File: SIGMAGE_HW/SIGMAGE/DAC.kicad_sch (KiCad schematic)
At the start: 80 parts, among them J20 SJ63073E, J21 SJ63073E, J24 SJ63073E, J25 SJ63073E, U10 PCM5102APWR, U20 PCM5102APWR, U21 PCM5102APWR, U3 PCM5102APWR

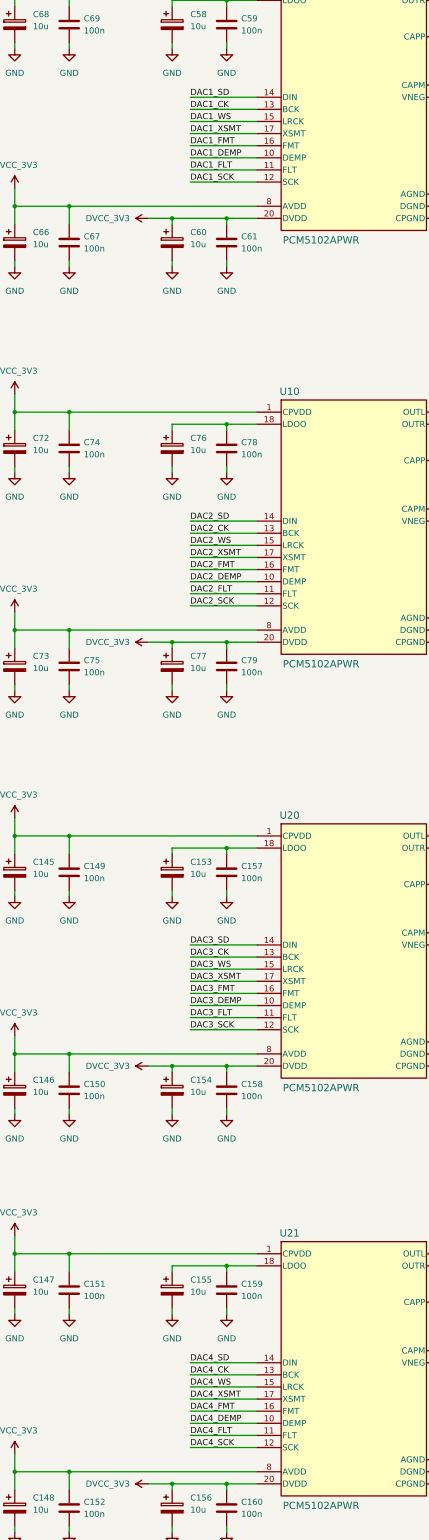
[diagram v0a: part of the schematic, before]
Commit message: finished schematic
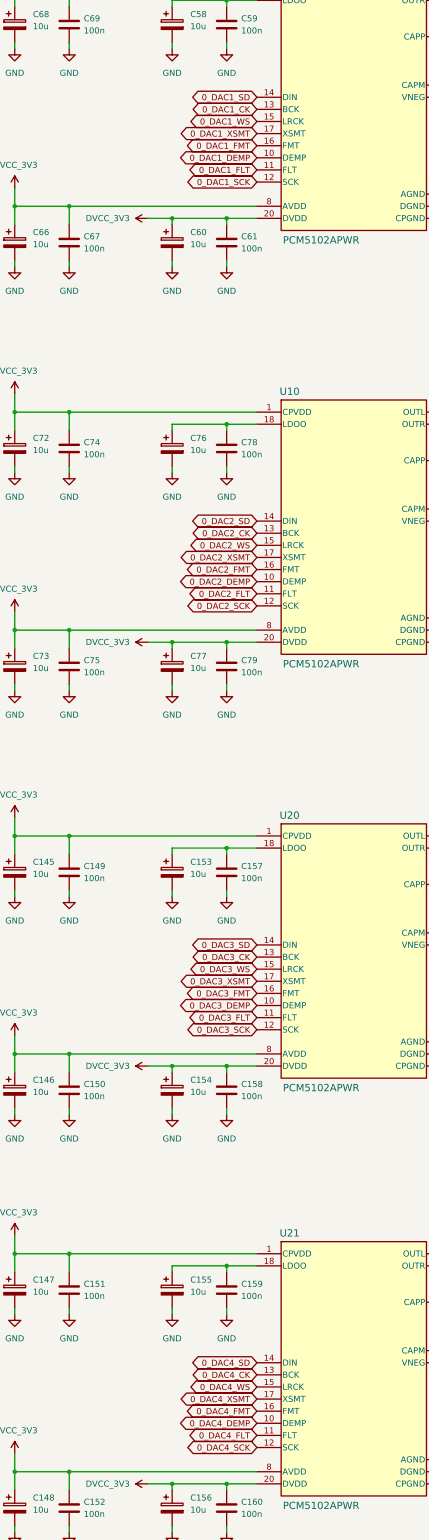
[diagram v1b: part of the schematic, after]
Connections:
- net DAC1_CK renamed 0_DAC1_CK
- net DAC1_DEMP renamed 0_DAC1_DEMP
- net DAC1_FLT renamed 0_DAC1_FLT
- net DAC1_FMT renamed 0_DAC1_FMT
- net DAC1_SCK renamed 0_DAC1_SCK
- net DAC1_SD renamed 0_DAC1_SD
- net DAC1_WS renamed 0_DAC1_WS
- net DAC1_XSMT renamed 0_DAC1_XSMT
- net DAC2_CK renamed 0_DAC2_CK
- net DAC2_DEMP renamed 0_DAC2_DEMP
- net DAC2_FLT renamed 0_DAC2_FLT
- net DAC2_FMT renamed 0_DAC2_FMT
- net DAC2_SCK renamed 0_DAC2_SCK
- net DAC2_SD renamed 0_DAC2_SD
- net DAC2_WS renamed 0_DAC2_WS
- net DAC2_XSMT renamed 0_DAC2_XSMT
- net DAC3_CK renamed 0_DAC3_CK
- net DAC3_DEMP renamed 0_DAC3_DEMP
- net DAC3_FLT renamed 0_DAC3_FLT
- net DAC3_FMT renamed 0_DAC3_FMT
- net DAC3_SCK renamed 0_DAC3_SCK
- net DAC3_SD renamed 0_DAC3_SD
- net DAC3_WS renamed 0_DAC3_WS
- net DAC3_XSMT renamed 0_DAC3_XSMT
- net DAC4_CK renamed 0_DAC4_CK
- net DAC4_DEMP renamed 0_DAC4_DEMP
- net DAC4_FLT renamed 0_DAC4_FLT
- net DAC4_FMT renamed 0_DAC4_FMT
- net DAC4_SCK renamed 0_DAC4_SCK
- net DAC4_SD renamed 0_DAC4_SD
- net DAC4_WS renamed 0_DAC4_WS
- net DAC4_XSMT renamed 0_DAC4_XSMT

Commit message: uga uga
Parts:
- C165, C166, C167, C168, C62, C63, C82, C83: footprint Capacitor_SMD:C_1206_3216Metric -> Resistor_SMD:R_0603_1608Metric
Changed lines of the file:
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@@
 			)
 		)
-		(property "Footprint" "Capacitor_SMD:C_1206_3216Metric"
+		(property "Footprint" "Resistor_SMD:R_0603_1608Metric"
 			(at 398.78 161.5948 0)
 			(hide yes)
@@
 			)
 		)
-		(property "Footprint" "Capacitor_SMD:C_1206_3216Metric"
+		(property "Footprint" "Resistor_SMD:R_0603_1608Metric"
 			(at 398.78 223.8248 0)
 			(hide yes)
@@
 			)
 		)
-		(property "Footprint" "Capacitor_SMD:C_1206_3216Metric"
+		(property "Footprint" "Resistor_SMD:R_0603_1608Metric"
 			(at 398.78 72.6948 0)
 			(hide yes)
@@
 			)
 		)
-		(property "Footprint" "Capacitor_SMD:C_1206_3216Metric"
+		(property "Footprint" "Resistor_SMD:R_0603_1608Metric"
 			(at 398.78 311.4548 0)
 			(hide yes)
@@
 			)
 		)
-		(property "Footprint" "Capacitor_SMD:C_1206_3216Metric"
+		(property "Footprint" "Resistor_SMD:R_0603_1608Metric"
 			(at 398.78 46.0248 0)
 			(hide yes)
@@
 			)
 		)
-		(property "Footprint" "Capacitor_SMD:C_1206_3216Metric"
+		(property "Footprint" "Resistor_SMD:R_0603_1608Metric"
 			(at 398.78 338.1248 0)
 			(hide yes)
@@
 			)
 		)
-		(property "Footprint" "Capacitor_SMD:C_1206_3216Metric"
+		(property "Footprint" "Resistor_SMD:R_0603_1608Metric"
 			(at 398.78 250.4948 0)
 			(hide yes)
@@
 			)
 		)
-		(property "Footprint" "Capacitor_SMD:C_1206_3216Metric"
+		(property "Footprint" "Resistor_SMD:R_0603_1608Metric"
 			(at 398.78 134.9248 0)
 			(hide yes)
